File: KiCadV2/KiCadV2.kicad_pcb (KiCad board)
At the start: 2 copper layers, 76.4 x 52.6 mm, 148 parts, among them J1 USB_C_Receptacle_PowerOnly_6P, J3 Screw_Terminal_01x02, J4 Screw_Terminal_01x02, U1 MT3608, U10 NC7SZ157P6X, U11 NC7SZ157P6X, U12 NC7SZ157P6X, U13 NC7SZ157P6X, U14 74LV08AT14-13, U15 HIP4080A, U16 NC7SZ157P6X, U17 MX3502S, U18 MX3502S, U2 74HC595, U22 DMHT10H032LFJ, U23 INA240A1D, U26 MX3502S, U3 NC7SZ157P6X, U30 DMHT10H032LFJ, U31 INA240A1D, U32 NC7SZ157P6X, U33 NC7SZ157P6X, U34 NC7SZ157P6X, U35 NC7SZ157P6X, U36 NC7SZ157P6X, U37 NC7SZ157P6X, U38 74LV08AT14-13, U39 HIP4080A, U4 NC7SZ157P6X, U40 MCP6002-xSN, U41 CJ432, U5 MX3502S, U6 NC7SZ157P6X, U7 DAC082S085CISDX/NOPB, U8 NC7SZ157P6X, U9 NC7SZ157P6X

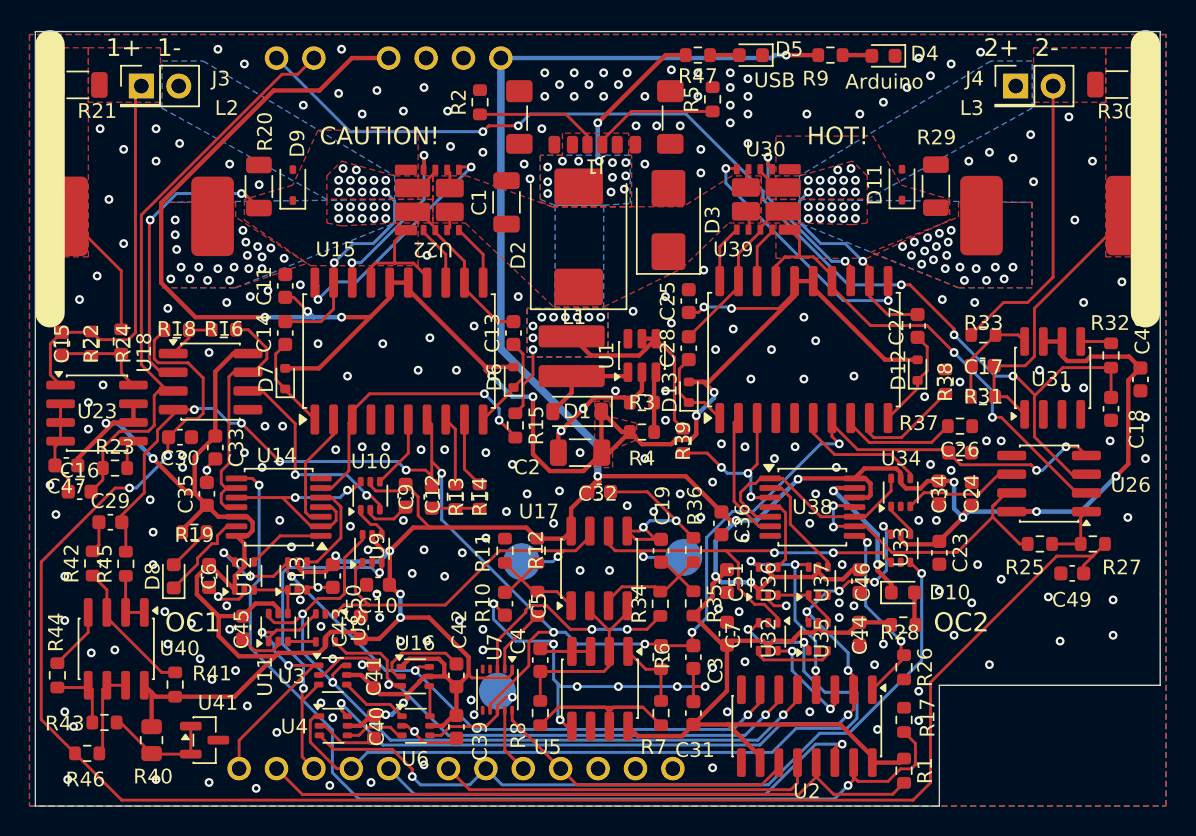
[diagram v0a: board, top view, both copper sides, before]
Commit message: goddammit forgot teardrops and final cleanup...
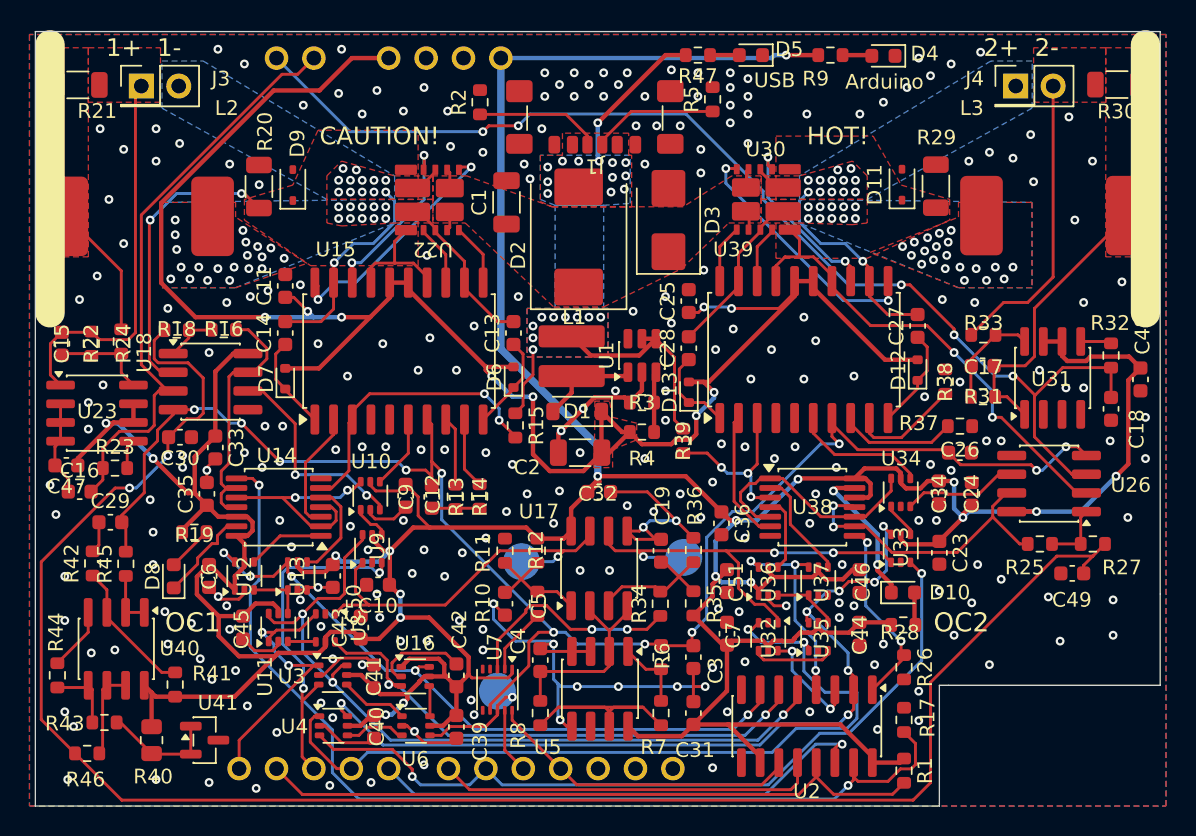
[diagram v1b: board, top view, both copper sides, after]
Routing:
- net +5V: track 346.3 -> 344.1 mm
- net GND: track 106.2 -> 104.2 mm
- net /VCM: track 109.8 -> 108.5 mm
- net Net-(U6-Z): track 8.23 -> 7.05 mm
- net /PerCoil1/OC_SENSE: track 32.3 -> 31.2 mm
- net /B1: track 37.3 -> 36.4 mm
- net /EN2: track 13.1 -> 12.2 mm
- net /PerCoil1/SignalProcessingChain/HF PWM: track 30.6 -> 29.8 mm
- net /PerCoil1/SignalProcessingChain/Current_Dir: track 7.88 -> 7.00 mm
- net /C1: track 46.3 -> 45.4 mm
- net /Vtri: track 13.7 -> 12.8 mm
- net Net-(U17B-+): track 10.5 -> 9.65 mm
- net /PerCoil/OC_SENSE: track 28.0 -> 27.1 mm
- net /PerCoil1/~{OC1}: track 21.3 -> 20.5 mm
- net /A1: track 53.1 -> 52.4 mm
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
